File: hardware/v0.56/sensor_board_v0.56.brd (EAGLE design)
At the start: 50.8 x 50.8 mm, 63 parts, among them J3 USB-MICROB, U10 TSL2591, U11 915MHz, U3 OPA344, U4 SI7021, U5 ATMEGA328P-MU, U6 ADMP401, U7 PMS7003, U8 MCP1703CB, U9 BMP280, X1 16 MHz

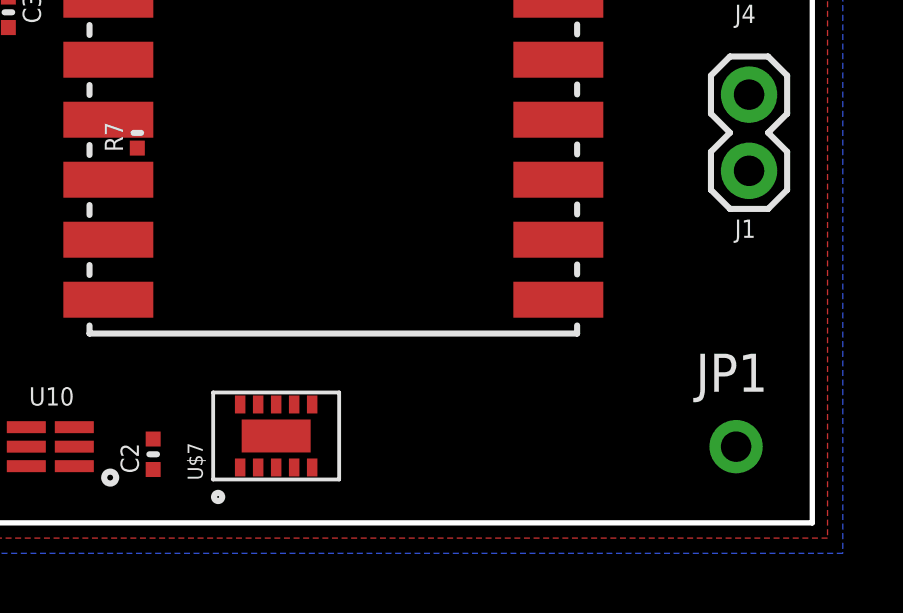
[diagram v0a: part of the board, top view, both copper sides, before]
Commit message: update
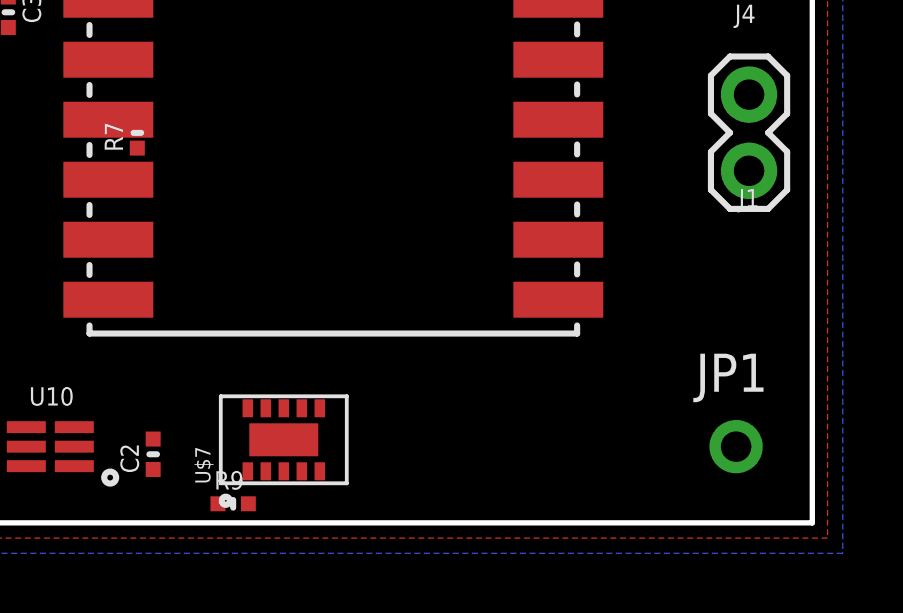
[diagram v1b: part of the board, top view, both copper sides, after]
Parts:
- added R9: 100K, Adafruit Feather 32u4 Bluefruit LE:MICROBUILDER__0402MP
- moved U$7 0.28 mm to (35.2, 1.42)
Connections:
- new net A1: U5.24
- new net A2: U5.25
- new net A3: U5.26
- new net A6: U5.19
- new net A7: U5.22
- new net N$13: R9.2, U$7.1
- net D5: now also U$7.7
- net GND: now also C2.1, J2.1, U$7.11
- net PWR: now also J2.2
- net SCL: now also U$7.10
- net SDA: now also U$7.9
- net VCC: now also C2.2, R9.1, U$7.6
